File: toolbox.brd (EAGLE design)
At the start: 100 x 80 mm, 75 parts, among them IC1 PIC18F4XK22PT, IC3 78L05SMD, T1 BC847, U2 AD654JRZ, U3 ADUM7441ARQZ

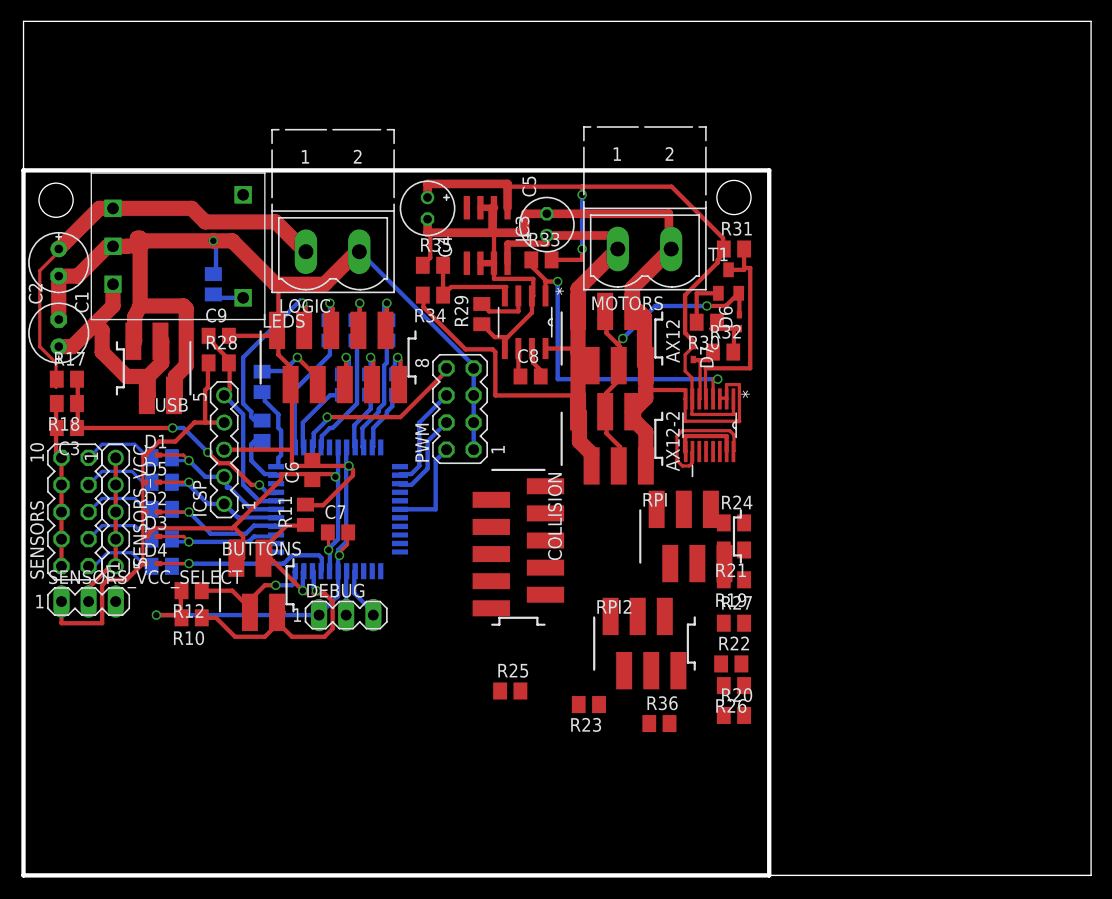
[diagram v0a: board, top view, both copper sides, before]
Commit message: WIP finished routing the board Removed useless datasheet
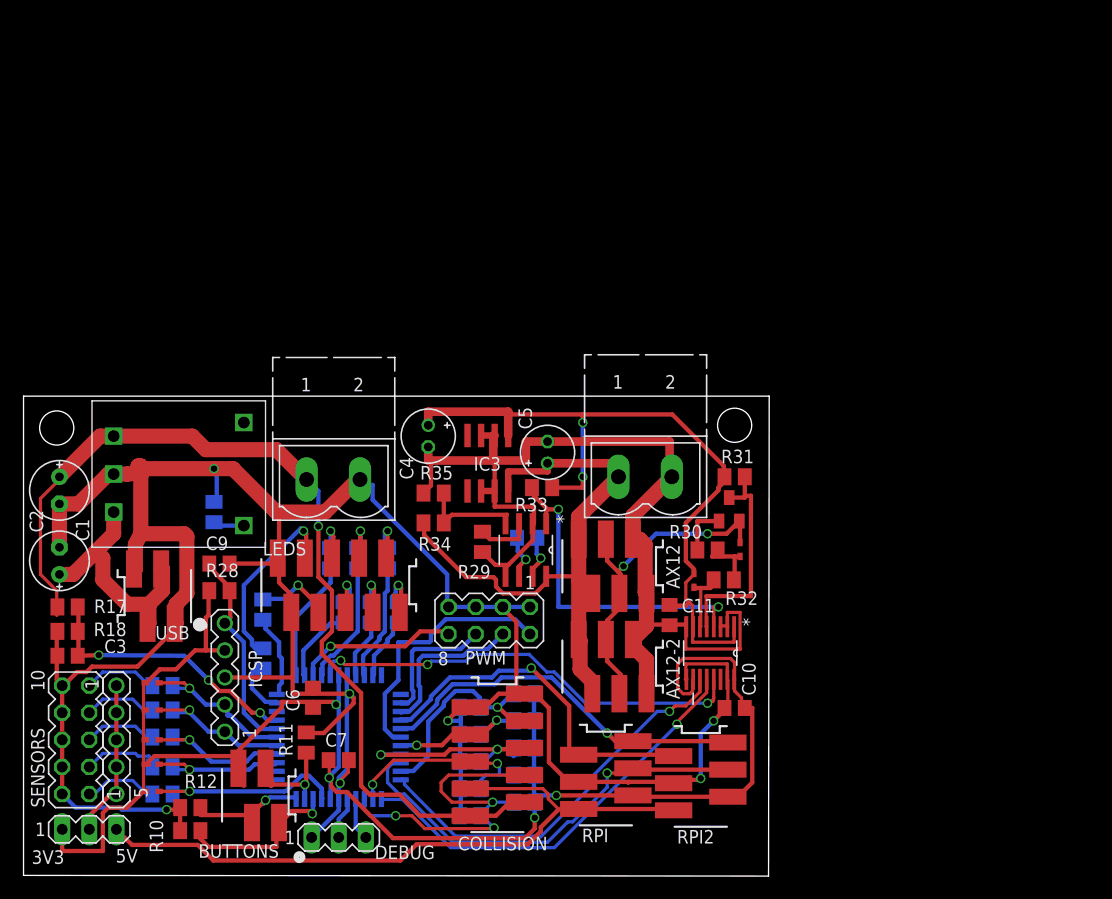
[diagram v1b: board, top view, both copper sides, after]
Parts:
- added C10, C11: 100n, rcl:C0805
- moved R19 33.1 mm to (41.8, 5.59), flipped to the bottom, turned to 0 degrees
- moved R21 31.7 mm to (41.8, 10.7), flipped to the bottom, turned to 0 degrees
- moved R24 27.0 mm to (46.9, 14.5), flipped to the bottom
- moved R27 25.8 mm to (46.9, 6.86), flipped to the bottom
- moved R20 25.6 mm to (41.8, 8.13), flipped to the bottom
- moved R22 24.8 mm to (41.8, 15.7), flipped to the bottom
- moved RPI 23.7 mm to (54.5, 9.40), turned to 90 degrees
- moved R26 21.3 mm to (46.9, 9.40), flipped to the bottom, turned to 0 degrees
- moved C1 21.3 mm to (3.37, 36.1)
- moved IC3 21.3 mm to (43.5, 38.6)
- moved AX12 21.3 mm to (55.2, 29.0)
- moved D2 21.3 mm to (12.0, 12.7)
- moved D4 21.3 mm to (12.0, 7.87)
- moved D6 21.3 mm to (67.1, 30.5)
- moved LEDS 21.3 mm to (29.5, 27.2)
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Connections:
- net GND: now also C10.2
- net N$67: now also C11.2
- net N$68: now also C11.1
- net VCC: now also C10.1
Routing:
- net GND: track 191.6 -> 264.1 mm, vias 4 -> 7
- net VCC: track 91.7 -> 158.5 mm, vias 2 -> 4
- net VDD: track 0.00 -> 66.0 mm
- net N$35: track 41.5 -> 90.1 mm, vias 0 -> 1
- net N$57: track 0.00 -> 41.6 mm, vias 0 -> 3
- net N$7: track 0.00 -> 40.7 mm, vias 0 -> 1
- net N$54: track 0.00 -> 40.4 mm, vias 0 -> 1
- net N$56: track 0.00 -> 37.8 mm, vias 0 -> 1
- net N$9: track 0.00 -> 35.4 mm, vias 0 -> 1
- net N$41: track 0.00 -> 34.2 mm, vias 0 -> 3
- net N$8: track 0.00 -> 33.8 mm, vias 0 -> 1
- net N$43: track 0.00 -> 22.9 mm, vias 0 -> 2
- net N$45: track 0.00 -> 20.9 mm, vias 0 -> 1
- net N$42: track 0.00 -> 19.8 mm, vias 0 -> 2
- net N$48: track 9.35 -> 24.6 mm
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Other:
- board size 100 x 80 mm -> 69.8 x 45 mm
- board text added: "3V3"
- board text added: "5V"
